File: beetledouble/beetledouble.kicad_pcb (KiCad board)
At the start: 4 copper layers, 31 x 59 mm, 50 parts, among them J1 XT30PW-M, J2 rxin, J4 motor_out, J5 motor_out, J6 prog connector, Q1 IPG20N04S4-12, Q2 IPG20N04S4-12, Q3 IPG20N04S4-12, Q4 IPG20N04S4-12, U1 78L12G-AB3-R, U2 DD4012SB, U3 ATtiny1614-SS, U4 NCP81155MNTXG, U5 NCP81155MNTXG, U6 NCP81155MNTXG, U7 NCP81155MNTXG

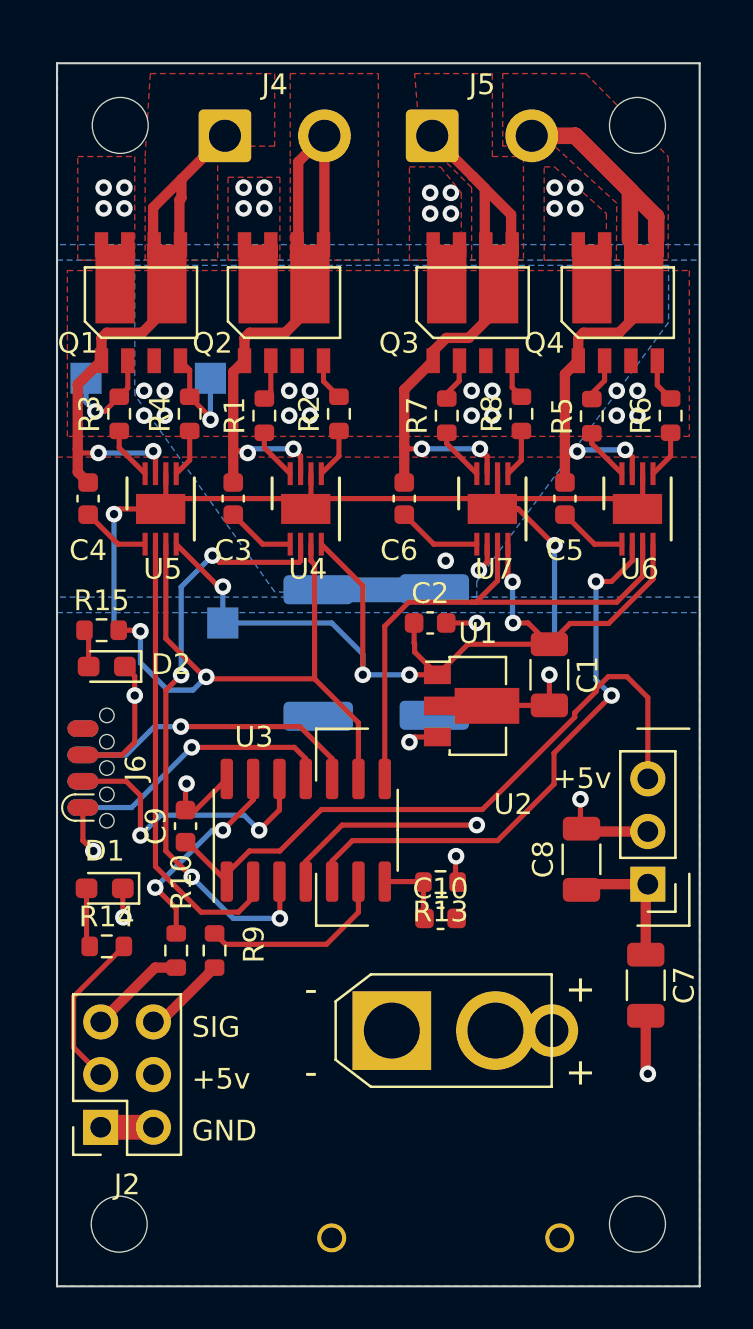
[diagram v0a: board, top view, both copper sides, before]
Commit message: Beetle esc
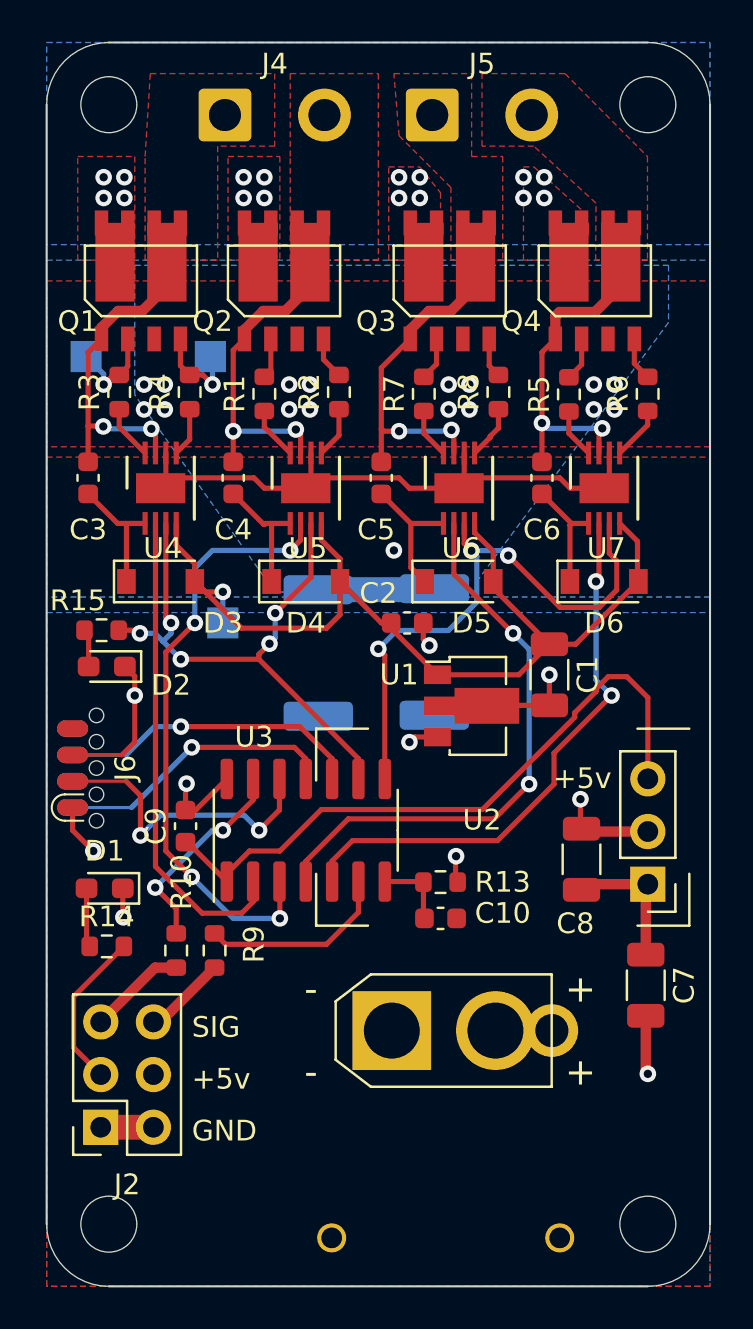
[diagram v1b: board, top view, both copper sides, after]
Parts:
- added D3: B5819W, Diode_SMD:D_SOD-123, F.Cu at (111.0, 97.0)
- added D4: B5819W, Diode_SMD:D_SOD-123, F.Cu at (118.0, 97.0)
- added D5: B5819W, Diode_SMD:D_SOD-123, F.Cu at (125.4, 97.0)
- added D6: B5819W, Diode_SMD:D_SOD-123, F.Cu at (132.4, 97.0)
- Q1, Q2, Q3, Q4: value IPG20N04S4-12 -> AON6884
- U4, U5, U6, U7: value NCP81155MNTXG -> ADP3110A
- moved U6 8.67 mm to (125.4, 92.5)
- moved U4 7.07 mm to (111.0, 92.5)
- moved U5 7.07 mm to (118.0, 92.5)
- moved U7 5.48 mm to (132.4, 92.5)
- moved R5 1.53 mm to (130.7, 88.0)
- moved Q4 1.53 mm to (131.9, 82.5)
- moved Q3 1.53 mm to (124.9, 82.5)
- moved R7 1.53 mm to (123.7, 88.0)
- moved R8 1.53 mm to (127.3, 87.9)
- moved R6 1.53 mm to (134.5, 88.0)
- moved C5 1.49 mm to (121.6, 92.0)
- moved C6 1.49 mm to (129.4, 92.0)
- moved H4 1.14 mm to (108.5, 74.0)
- moved H3 1.12 mm to (134.5, 74.0)
- moved C2 1.11 mm to (122.9, 99.0)
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- renumbered C4 to C3, C3 to C4, C6 to C5, C5 to C6
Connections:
- C3 pad 1: Net-(C4-Pad1) -> /driver1/BOOST1
- C4 pad 1: Net-(C3-Pad1) -> /driver1/BOOST2
- C5 pad 1: Net-(C6-Pad1) -> /driver2/BOOST1
- C6 pad 1: Net-(C5-Pad1) -> /driver2/BOOST2
- U4 pad 1: Net-(C3-Pad1) -> /driver1/BOOST1
- U4 pad 2: MOTORR_1 -> MOTORF_1
- U4 pad 5: /driver1/MOTORL2 -> /driver1/MOTORL1
- U4 pad 7: /driver1/MOTORS2 -> /driver1/MOTORS1
- U4 pad 8: /driver1/MOTORH2 -> /driver1/MOTORH1
- U5 pad 1: Net-(C4-Pad1) -> /driver1/BOOST2
- U5 pad 2: MOTORF_1 -> MOTORR_1
- U5 pad 5: /driver1/MOTORL1 -> /driver1/MOTORL2
- U5 pad 7: /driver1/MOTORS1 -> /driver1/MOTORS2
- U5 pad 8: /driver1/MOTORH1 -> /driver1/MOTORH2
- U6 pad 1: Net-(C5-Pad1) -> /driver2/BOOST1
- U6 pad 2: MOTORR_2 -> MOTORF_2
- U6 pad 5: /driver2/MOTORL2 -> /driver2/MOTORL1
- U6 pad 7: /driver2/MOTORS2 -> /driver2/MOTORS1
- U6 pad 8: /driver2/MOTORH2 -> /driver2/MOTORH1
- U7 pad 1: Net-(C6-Pad1) -> /driver2/BOOST2
- U7 pad 2: MOTORF_2 -> MOTORR_2
- U7 pad 5: /driver2/MOTORL1 -> /driver2/MOTORL2
- U7 pad 7: /driver2/MOTORS1 -> /driver2/MOTORS2
- U7 pad 8: /driver2/MOTORH1 -> /driver2/MOTORH2
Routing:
- net GND: track 77.6 -> 59.9 mm, vias 9 -> 7
- net /driver2/MOTORS2: track 32.1 -> 16.5 mm
- net /driver1/MOTORS2: track 28.3 -> 16.1 mm
- net /driver1/MOTORS1: track 28.0 -> 16.2 mm
- net /driver2/MOTORS1: track 27.6 -> 16.7 mm
- net /driver2/BOOST1: track 0.00 -> 6.67 mm
- net /driver1/BOOST2: track 0.00 -> 6.20 mm
- net /driver1/BOOST1: track 0.00 -> 6.16 mm
- net /driver2/BOOST2: track 0.00 -> 5.67 mm
- net Net-(C6-Pad1): track 4.09 -> 0.00 mm
- net Net-(C4-Pad1): track 3.34 -> 0.00 mm
- net Net-(C3-Pad1): track 3.34 -> 0.00 mm
- net Net-(C5-Pad1): track 3.34 -> 0.00 mm
- net MOTORF_2: track 24.3 -> 27.4 mm
- net MOTOR_ENABLE_1: track 31.5 -> 28.6 mm, vias 2 -> 5
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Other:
- board size 31 x 59 mm -> 32 x 60 mm
